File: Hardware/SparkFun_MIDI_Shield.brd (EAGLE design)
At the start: 59.7 x 53.3 mm, 34 parts, among them J1 MIDI IN, J2 MIDI OUT, J3 UNO_R3_SHIELD, U2 74AHC1G125

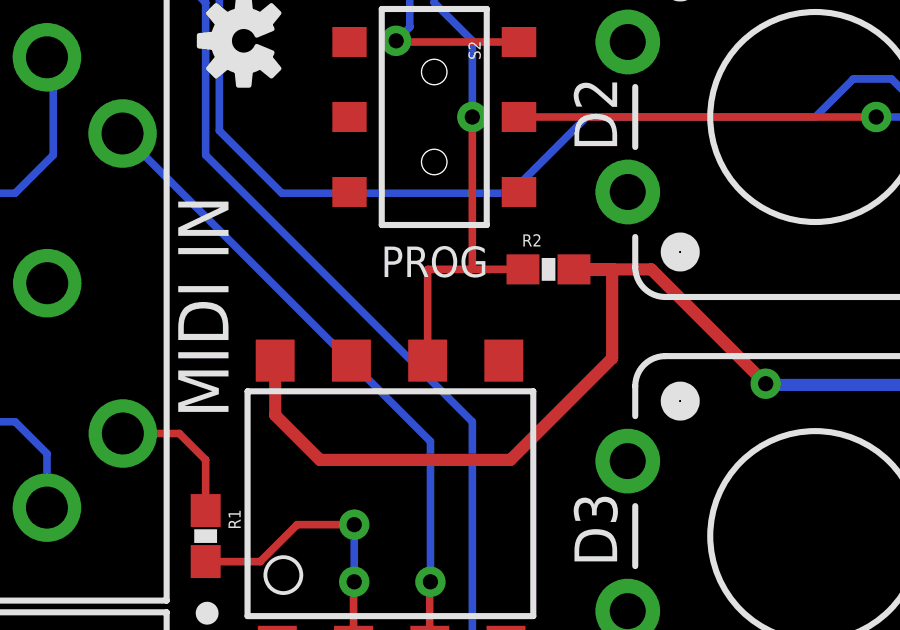
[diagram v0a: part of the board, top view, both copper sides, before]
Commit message: Updates after QC checklist.
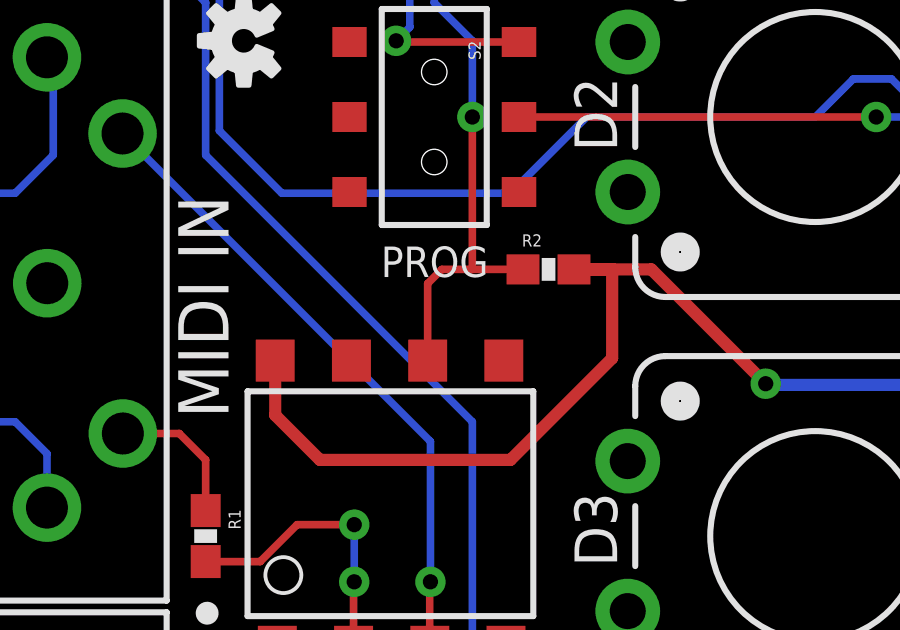
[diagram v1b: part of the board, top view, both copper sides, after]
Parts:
- renumbered U$1 to U1
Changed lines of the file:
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@@
 <layer number="18" name="Vias" color="2" fill="1" visible="yes" active="yes"/>
 <layer number="19" name="Unrouted" color="6" fill="1" visible="yes" active="yes"/>
-<layer number="20" name="Dimension" color="15" fill="1" visible="yes" active="yes"/>
+<layer number="20" name="Dimension" color="15" fill="1" visible="no" active="yes"/>
 <layer number="21" name="tPlace" color="16" fill="1" visible="yes" active="yes"/>
-<layer number="22" name="bPlace" color="14" fill="1" visible="yes" active="yes"/>
+<layer number="22" name="bPlace" color="14" fill="1" visible="no" active="yes"/>
 <layer number="23" name="tOrigins" color="15" fill="1" visible="yes" active="yes"/>
-<layer number="24" name="bOrigins" color="15" fill="1" visible="yes" active="yes"/>
+<layer number="24" name="bOrigins" color="15" fill="1" visible="no" active="yes"/>
 <layer number="25" name="tNames" color="7" fill="1" visible="no" active="yes"/>
 <layer number="26" name="bNames" color="7" fill="1" visible="no" active="yes"/>
@@
 <attribute name="PROD_ID" value="SWCH-08179" x="25.4" y="40.64" size="1.778" layer="27" font="vector" ratio="15" rot="R270" display="off"/>
 </element>
-<element name="U$1" library="SparkFun-DiscreteSemi" package="8-SMD" value="6N138M" x="24.13" y="27.94">
-<attribute name="PROD_ID" value="IC-09482" x="24.13" y="27.94" size="1.778" layer="27" font="vector" ratio="15" display="off"/>
-</element>
 <element name="JP3" library="SparkFun-Passives" package="PAD-JUMPER-2-NO_YES_SILK" value="JUMPER-PAD-2-NOYES_SILK" x="8.89" y="16.51" rot="MR180"/>
 <element name="JP4" library="SparkFun-Passives" package="PAD-JUMPER-2-NO_YES_SILK" value="JUMPER-PAD-2-NOYES_SILK" x="8.89" y="8.89" rot="MR180"/>
@@
 <element name="SJ1" library="SparkFun-Passives" package="PAD-JUMPER-3-2OF3_NC_BY_TRACE_YES_SILK_FULL_BOX" value="TX sel" x="25.4" y="45.72" rot="MR0"/>
 <element name="SJ2" library="SparkFun-Passives" package="PAD-JUMPER-3-2OF3_NC_BY_TRACE_YES_SILK_FULL_BOX" value="RX sel" x="19.05" y="45.72" rot="MR0"/>
+<element name="U1" library="SparkFun-DiscreteSemi" package="8-SMD" value="6N138M" x="24.13" y="27.94">
+<attribute name="PROD_ID" value="IC-09482" x="24.13" y="27.94" size="1.778" layer="27" font="vector" ratio="15" display="off"/>
+</element>
 </elements>
 <signals>
@@
 <contactref element="U2" pad="1"/>
 <contactref element="S1" pad="1"/>
-<contactref element="U$1" pad="5"/>
 <contactref element="JP3" pad="1"/>
 <contactref element="JP1" pad="1"/>
+<contactref element="U1" pad="5"/>
 </signal>
 <signal name="VCC">
@@
 <wire x1="30.06" y1="35.56" x2="32.639" y2="35.56" width="0.4064" layer="1"/>
 <wire x1="32.639" y1="35.56" x2="36.449" y2="31.75" width="0.4064" layer="1"/>
-<contactref element="U$1" pad="8"/>
-<wire x1="20.1" y1="32.52" x2="20.1" y2="30.7" width="0.4064" layer="1"/>
 <wire x1="20.1" y1="30.7" x2="21.59" y2="29.21" width="0.4064" layer="1"/>
 <wire x1="21.59" y1="29.21" x2="27.94" y2="29.21" width="0.4064" layer="1"/>
@@
 <wire x1="19.685" y1="16.6061" x2="19.685" y2="14.605" width="0.4064" layer="1"/>
 <wire x1="19.685" y1="14.605" x2="20.32" y2="13.97" width="0.4064" layer="1"/>
+<contactref element="U1" pad="8"/>
+<wire x1="20.1" y1="32.52" x2="20.1" y2="30.7" width="0.4064" layer="1"/>
 </signal>
 <signal name="56">
@@
 <wire x1="22.71" y1="21.994" x2="24.52" y2="20.184" width="0.254" layer="1"/>
 <wire x1="17.78" y1="25.82" x2="19.597" y2="25.82" width="0.254" layer="1"/>
-<contactref element="U$1" pad="2"/>
+<contactref element="U1" pad="2"/>
 <wire x1="22.71" y1="22.98" x2="22.71" y2="21.994" width="0.254" layer="1"/>
 <wire x1="22.71" y1="22.98" x2="22.71" y2="25.123" width="0.254" layer="1"/>
@@
 <wire x1="28.829" y1="19.059" x2="28.82" y2="19.05" width="0.254" layer="1"/>
 <wire x1="25.273" y1="29.827" x2="15.01" y2="40.09" width="0.254" layer="16"/>
-<contactref element="U$1" pad="3"/>
+<contactref element="U1" pad="3"/>
+<wire x1="25.25" y1="22.98" x2="25.25" y2="21.867" width="0.254" layer="1"/>
 <wire x1="25.25" y1="22.98" x2="25.25" y2="25.123" width="0.254" layer="1"/>
 <wire x1="25.25" y1="25.123" x2="25.273" y2="25.146" width="0.254" layer="1"/>
-<wire x1="25.25" y1="22.98" x2="25.25" y2="21.867" width="0.254" layer="1"/>
 </signal>
 <signal name="PORT-RX">
 <contactref element="R2" pad="1"/>
-<contactref element="U$1" pad="6"/>
-<wire x1="25.18" y1="32.52" x2="25.18" y2="35.56" width="0.254" layer="1"/>
 <wire x1="28.36" y1="35.56" x2="26.67" y2="35.56" width="0.254" layer="1"/>
 <contactref element="SJ1" pad="2"/>
@@
 <wire x1="26.67" y1="43.18" x2="26.67" y2="40.64" width="0.254" layer="16"/>
 <wire x1="26.67" y1="40.64" x2="26.67" y2="35.56" width="0.254" layer="1"/>
-<wire x1="26.67" y1="35.56" x2="25.18" y2="35.56" width="0.254" layer="1"/>
 <via x="26.67" y="40.64" extent="1-16" drill="0.508"/>
+<wire x1="25.18" y1="35.086" x2="25.654" y2="35.56" width="0.254" layer="1"/>
+<wire x1="25.654" y1="35.56" x2="26.67" y2="35.56" width="0.254" layer="1"/>
+<contactref element="U1" pad="6"/>
+<wire x1="25.18" y1="32.52" x2="25.18" y2="35.086" width="0.254" layer="1"/>
 </signal>
 <signal name="1235">

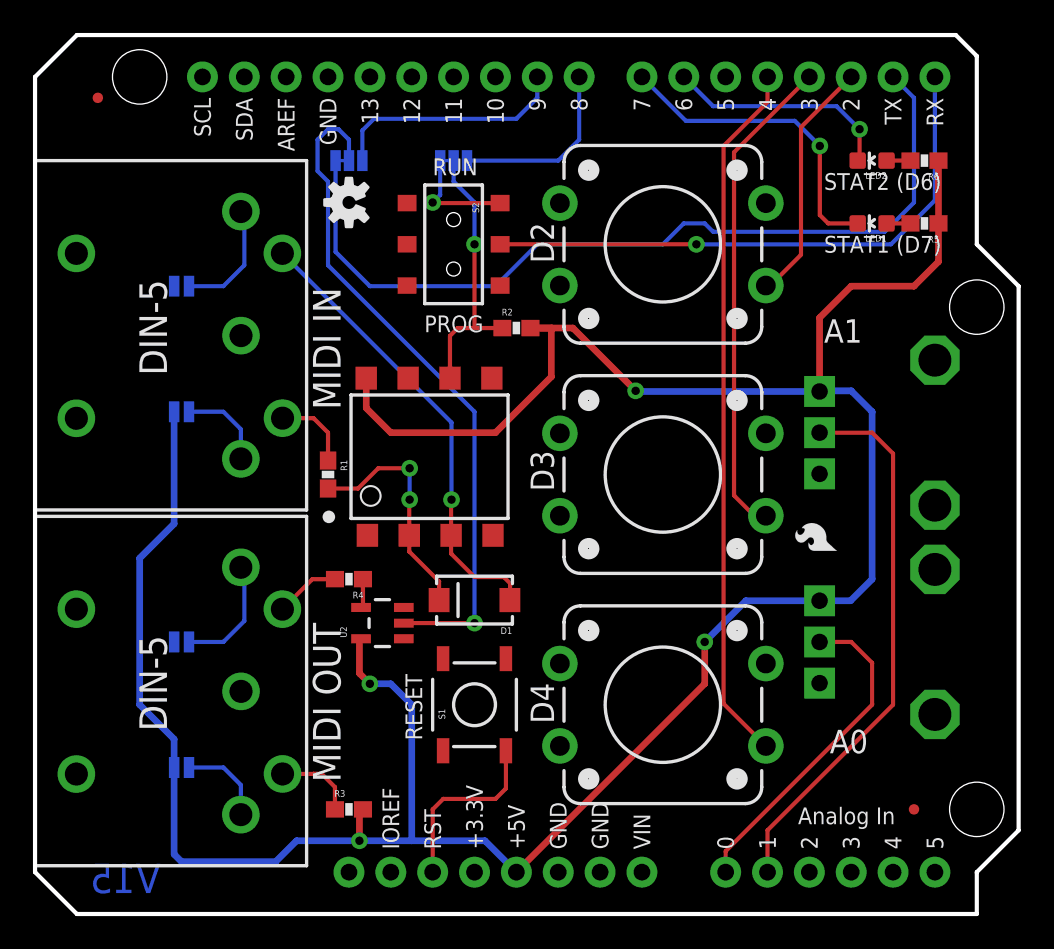
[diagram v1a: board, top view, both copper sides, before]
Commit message: Prototype Revisions WIP
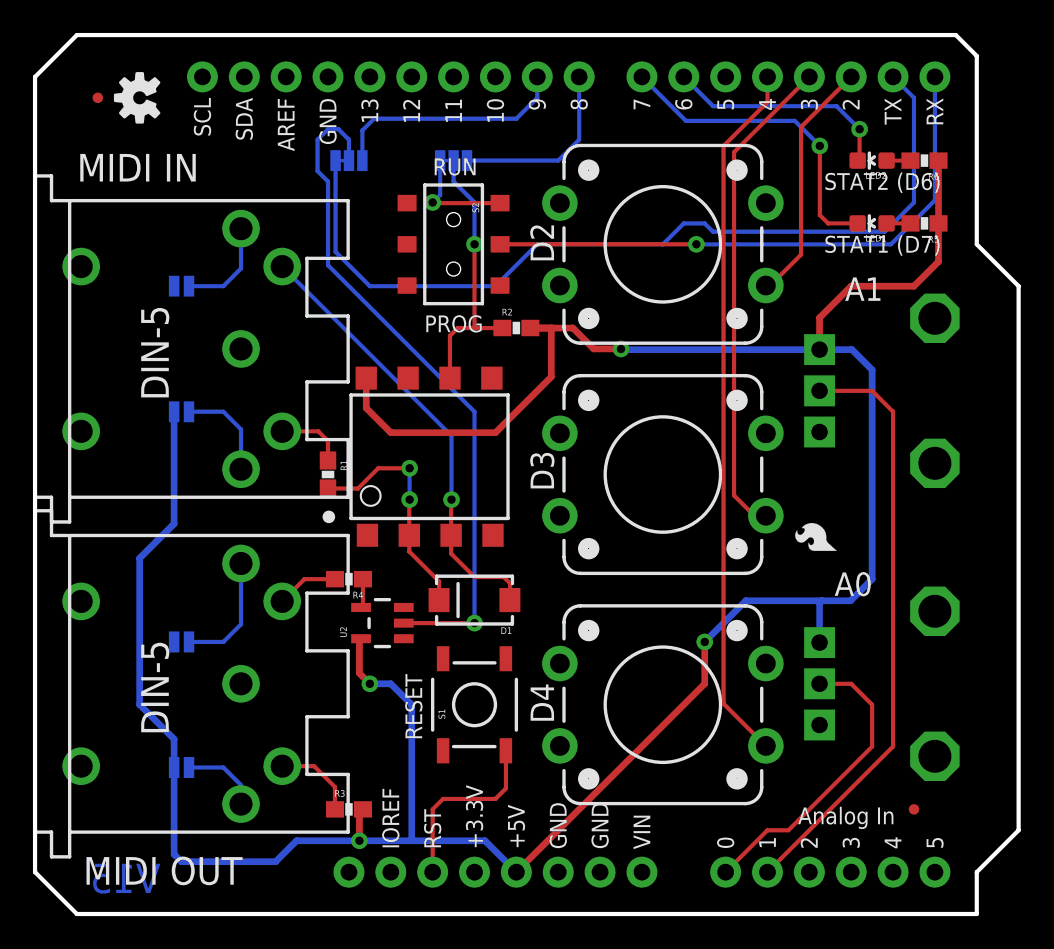
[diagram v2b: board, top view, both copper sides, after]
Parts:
- J1, J2: device Testing:5-PIN-DIN-RA-PCB -> Testing:5-PIN-DIN-RA-PCB-NEW
- J3: device Testing:UNO_R3_SHIELD_HOLES -> SparkFun-Boards:UNO_R3_SHIELD
- moved LOGO2 14.2 mm to (6.35, 49.5)
- moved J1 8.98 mm to (0.00, 34.3)
- moved J2 8.89 mm to (0.00, 14.0)
- moved RV2 2.54 mm to (54.6, 14.0)
- moved RV1 2.54 mm to (54.6, 31.8)
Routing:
- net A1: track 33.5 -> 36.1 mm
- net A0: track 20.1 -> 18.3 mm
- net N$6: track 7.23 -> 6.02 mm
- net VCC: track 171.1 -> 172.0 mm
- net PIN5: track 27.8 -> 27.0 mm
- net N$5: track 5.39 -> 4.75 mm
- net N$7: track 5.39 -> 6.02 mm
- net N$2: track 4.81 -> 4.21 mm
